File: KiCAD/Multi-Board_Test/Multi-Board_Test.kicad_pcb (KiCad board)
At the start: 2 copper layers, 189.2 x 95.9 mm, 21 parts, among them J1 XW4M-10D2-H1DS, J2 XW4M-10D2-H1DS, J3 XW4M-02D1-H1DA

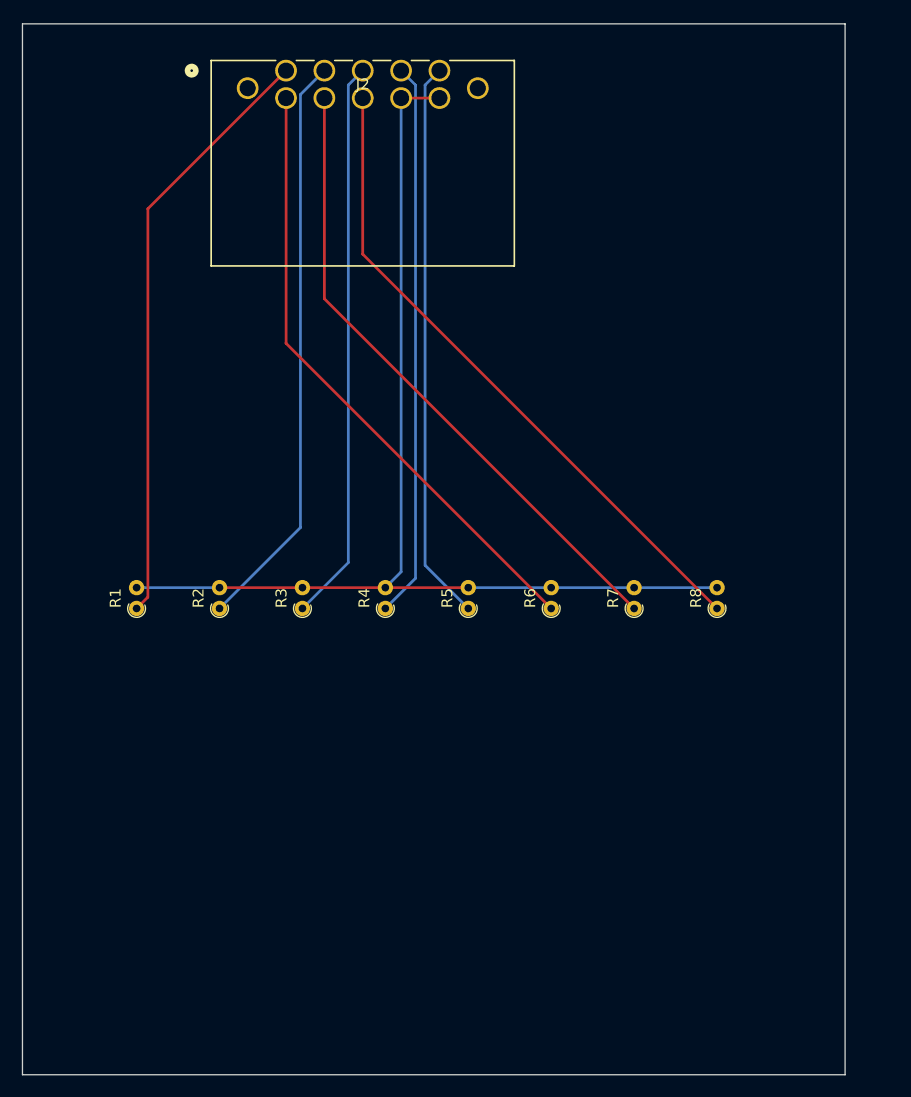
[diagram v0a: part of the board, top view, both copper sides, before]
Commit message: Worked on multi board workflow
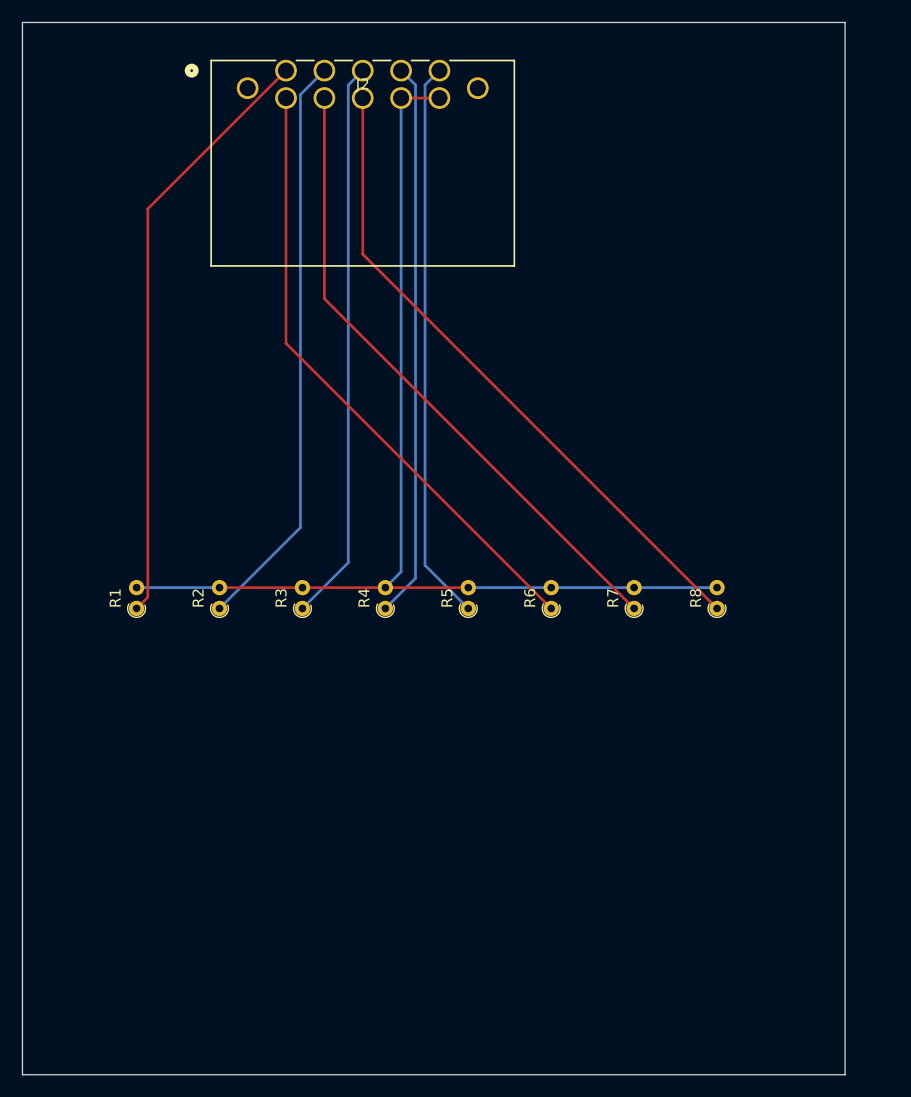
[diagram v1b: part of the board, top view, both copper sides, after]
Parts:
- moved B1 3.56 mm to (36.3, 34.2)
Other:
- board size 189.2 x 95.9 mm -> 189.2 x 96 mm
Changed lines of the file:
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@@
   )
   (footprint "PCM_kikit:Board" (layer "F.Cu")
-    (at 39.878 34.163)
+    (at 36.322 34.163)
     (descr "Mark board for extraction")
-    (attr board_only exclude_from_pos_files exclude_from_bom allow_missing_courtyard)
+    (attr through_hole)
     (fp_text reference "B1" (at -4.5 -5) (layer "Dwgs.User")
         (effects (font (size 1 1) (thickness 0.15)) (justify left))
@@
   (gr_rect (start 155.321 34.9885) (end 225.298 128.397)
     (stroke (width 0.1) (type default)) (fill none) (layer "Edge.Cuts"))
-  (gr_rect (start 36.068 34.29) (end 111.125 130.175)
+  (gr_rect (start 36.068 34.163) (end 111.125 130.175)
     (stroke (width 0.1) (type default)) (fill none) (layer "Edge.Cuts"))
   (segment (start 160.75 46.721998) (end 160.75 86.239) (width 0.25) (layer "F.Cu") (net 1))
